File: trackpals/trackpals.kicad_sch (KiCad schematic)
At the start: 103 parts, among them J1 CONUFL001-SMD-T, J2 Conn_01x02_Socket, J3 Battery Connector, J4 CONUFL001-SMD-T, Q1 BC848, Q2 AO4459, Q3 BSS138, Q4 BSS138, SW1 SW_Push, SW2 SW_Push, SW3 SW_Push, U1 TXS0102DCT, U2 BQ24040DSQR, U3 TPS73733DCQR, U4 TPL5110, U5 CH340C, U6 SIM800C, U7 ESP32-WROOM-32, U8 NEO-6M-GPS, U9 HK24C32HA-USR-B

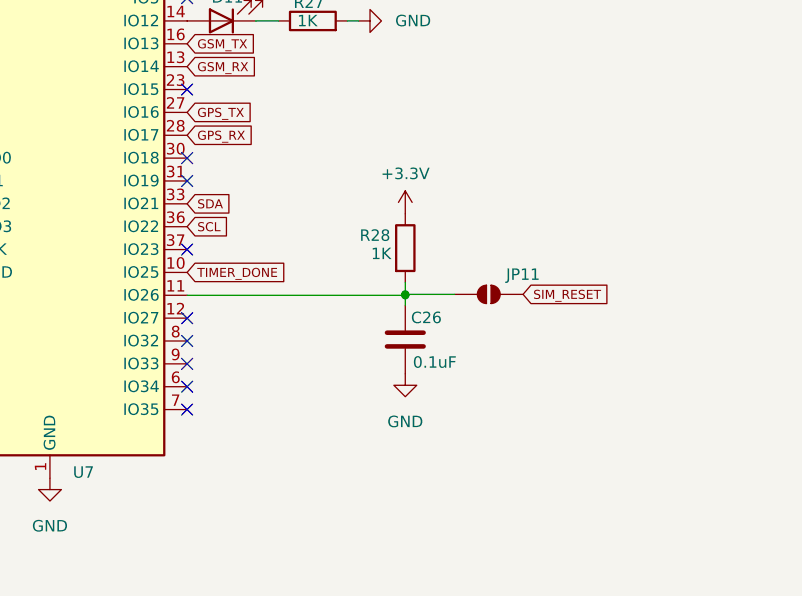
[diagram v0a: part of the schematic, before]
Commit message: - DONE PCB
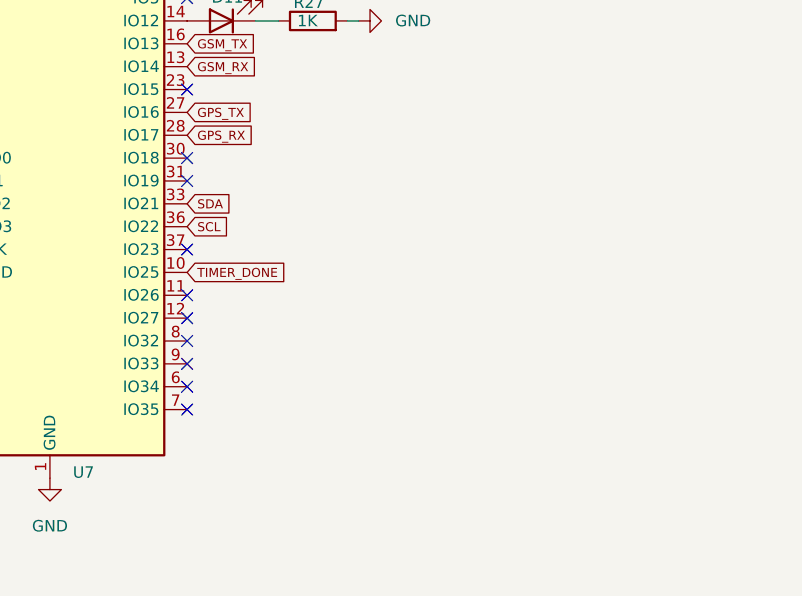
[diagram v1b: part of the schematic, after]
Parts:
- removed C26: 0.1uF, Capacitor_SMD:C_0805_2012Metric_Pad1.18x1.45mm_HandSolder, symbol Device:C
- removed JP11: SolderJumper_2_Open, Jumper:SolderJumper-2_P1.3mm_Open_Pad1.0x1.5mm, symbol Jumper:SolderJumper_2_Open
- removed R28: 1K, Resistor_SMD:R_0603_1608Metric_Pad0.98x0.95mm_HandSolder, symbol Device:R
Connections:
- no-connect marks 59 -> 60

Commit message: updated tssop
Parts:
- C7: LCSC (none) -> C15850
- D12: footprint Diode_THT:D_DO-41_SOD81_P10.16mm_Horizontal -> Diode_SMD:D_SOD-123F; LCSC (none) -> C2892326
- D6: LCSC (none) -> C2297
- J4: LCSC (none) -> C5137195
- L1: LCSC (none) -> C2885873
- Q2: LCSC (none) -> C49047
- R13: LCSC C105578 -> C25804
- U4: LCSC (none) -> C2651358
- U9: footprint Footprint_track:SOP-8_L5.0-W4.0-P1.27-LS6.2-BL -> Package_SO:TSSOP-8_4.4x3mm_P0.65mm; LCSC (none) -> C33576253
